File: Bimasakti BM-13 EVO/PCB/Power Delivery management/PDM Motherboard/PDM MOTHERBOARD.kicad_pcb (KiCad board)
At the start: 2 copper layers, 107.9 x 103.1 mm, 32 parts

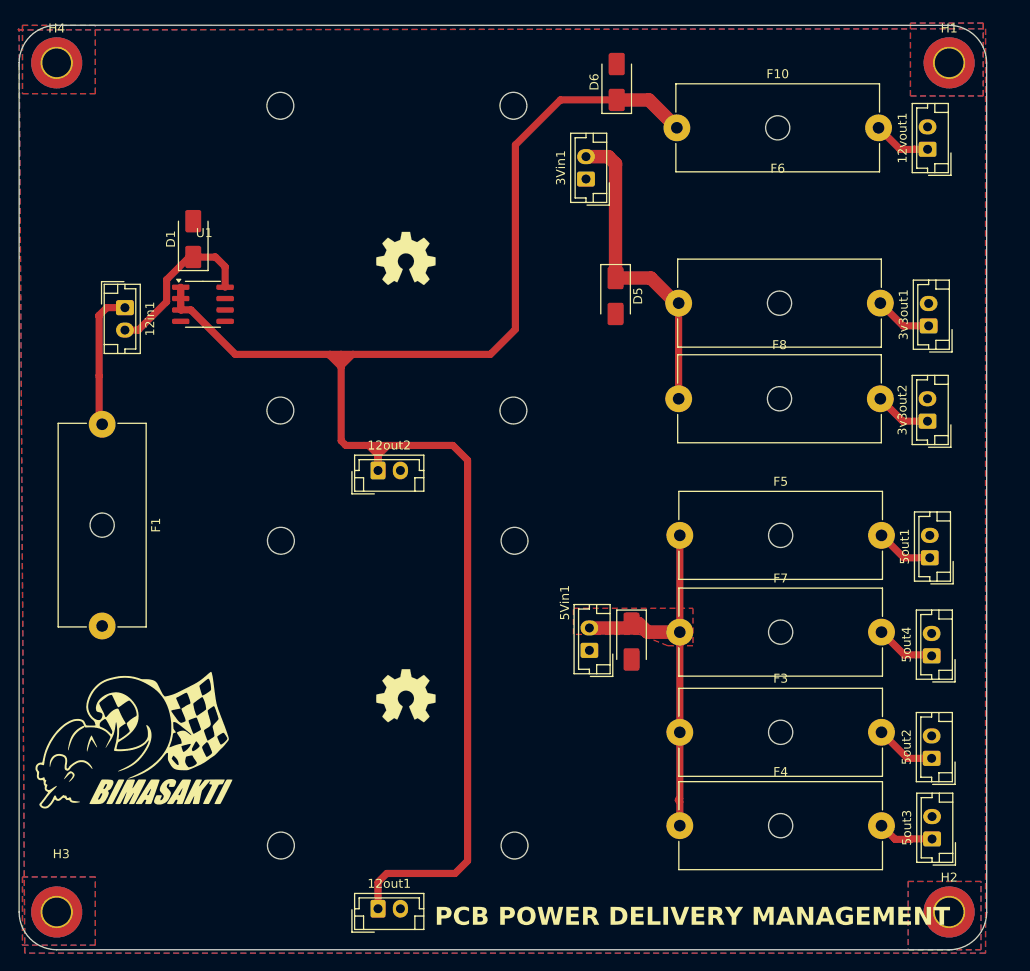
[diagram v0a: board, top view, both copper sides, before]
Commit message: ngecilin pdm
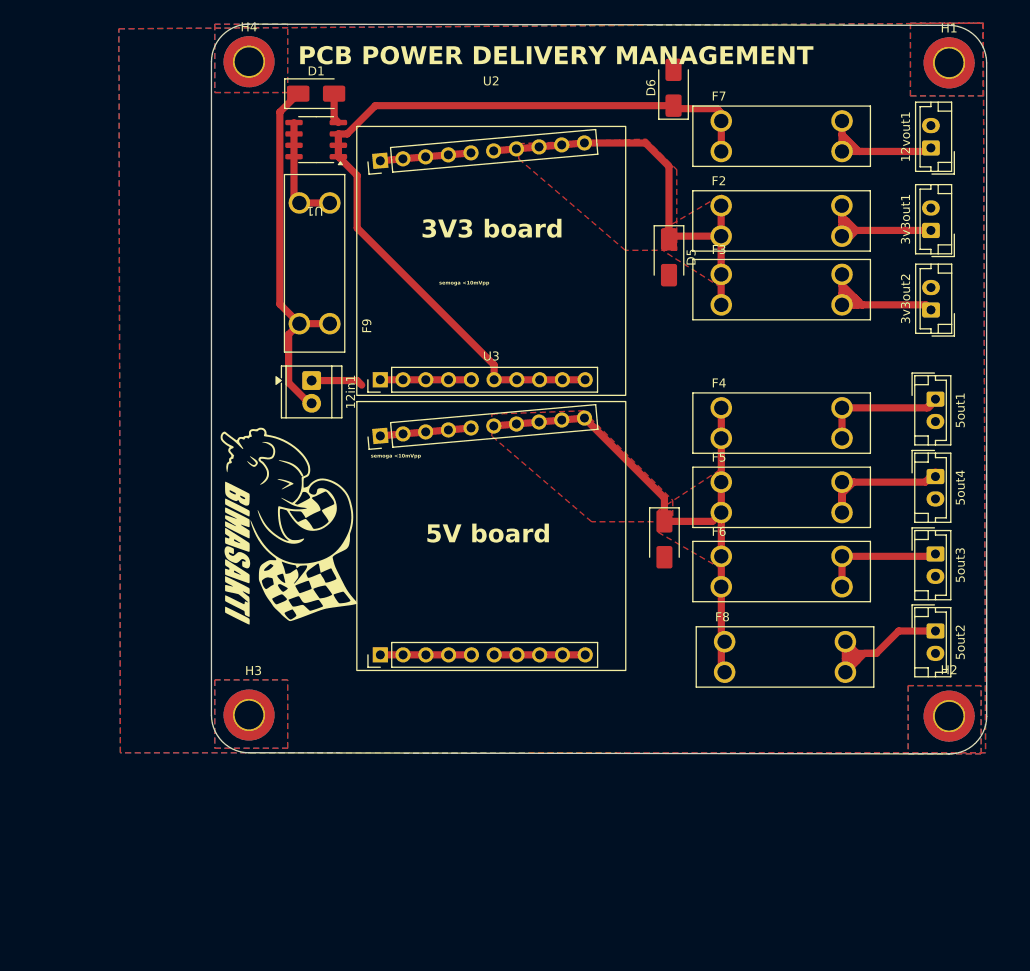
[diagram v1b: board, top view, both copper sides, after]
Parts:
- removed 12out1, 12out2, 3Vin1, 5Vin1: ~, Connector_JST:JST_EH_B2B-EH-A_1x02_P2.50mm_Vertical
- removed F1, F10: 1A, Fuse:Fuseholder_Cylinder-5x20mm_Schurter_0031_8201_Horizontal_Open
- removed N1: pdm 3.3V, Symbol:OSHW-Symbol_6.7x6mm_SilkScreen
- removed N2: pdm 5v, Symbol:OSHW-Symbol_6.7x6mm_SilkScreen
- added F2: 3557-2, 0_FUSE:0_FUSE_3557-2, F.Cu at (134.7, 37.1)
- added F9: 3557-2, 0_FUSE:0_FUSE_3557-2, F.Cu at (82.6, 41.8)
- added U2: ~, BIMS_BUCK:BIMS_BUCK, F.Cu at (102.3, 22.0)
- added U3: ~, BIMS_BUCK:BIMS_BUCK, F.Cu at (102.3, 52.7)
- 12in1: footprint Connector_JST:JST_EH_B2B-EH-A_1x02_P2.50mm_Vertical -> TerminalBlock_TE-Connectivity:TerminalBlock_TE_282834-2_1x02_P2.54mm_Horizontal
- F3, F4, F5, F6, F7, F8: value 1A -> 3557-2; footprint Fuse:Fuseholder_Cylinder-5x20mm_Schurter_0031_8201_Horizontal_Open -> 0_FUSE:0_FUSE_3557-2
- moved F7 56.5 mm to (134.7, 27.6)
- moved F3 50.7 mm to (134.7, 44.7)
- moved F4 46.3 mm to (134.7, 59.6)
- moved F6 32.1 mm to (134.7, 76.2)
- moved 5out3 31.8 mm to (151.9, 74.2), turned to -90 degrees
- moved F8 31.2 mm to (135.1, 85.7)
- moved H3 30.7 mm to (75.3, 92.2)
- moved G*** 29.5 mm to (79.8, 71.1), turned to -90 degrees
- moved 12in1 22.4 mm to (82.3, 54.9)
- moved H2 21.8 mm to (153.4, 92.3)
- moved H4 21.5 mm to (75.3, 19.3)
- moved D1 21.2 mm to (82.8, 22.9), turned to 0 degrees
- moved 5out4 20.0 mm to (151.9, 65.6), turned to -90 degrees
- moved 5out1 17.7 mm to (151.9, 56.9), turned to -90 degrees
- moved 5out2 14.2 mm to (151.9, 82.8), turned to -90 degrees
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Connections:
- U1 pad 1: Net-(12in1-Pin_2) -> Net-(U1-D)
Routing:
- net +12: track 179.6 -> 104.4 mm
- net GND: track 16.0 -> 49.9 mm
- net Net-(12in1-Pin_2): track 18.7 -> 41.4 mm
- net Net-(5out2-Pin_1): track 6.80 -> 27.5 mm
- net 5Vin: track 42.5 -> 61.8 mm
- net Net-(3v3out2-Pin_1): track 6.30 -> 20.1 mm
- net Net-(3v3out1-Pin_1): track 6.44 -> 19.6 mm
- net Net-(U1-D): track 0.00 -> 12.6 mm
- net Net-(5out4-Pin_1): track 6.69 -> 18.2 mm
- net 3Vin: track 35.6 -> 46.0 mm
- net Net-(12vout1-Pin_1): track 6.48 -> 16.6 mm
- net Net-(5out1-Pin_1): track 6.42 -> 14.6 mm
- net Net-(5out3-Pin_1): track 6.29 -> 14.0 mm
- added copper zone on F.Cu, net 3Vin
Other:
- board size 107.9 x 103.1 mm -> 86.5 x 81.4 mm
- board text added: "3V3 board"
- board text added: "5V board"
- board text added: "semoga <10mVpp"
